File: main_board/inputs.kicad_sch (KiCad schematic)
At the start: 49 parts, among them J16 3.5mm Jack, J17 3.5mm Jack, U10 TLV2172IDR, U11 MCP3021, U12 TLV2172IDR, U13 MCP3021, U19 TLV2172IDR

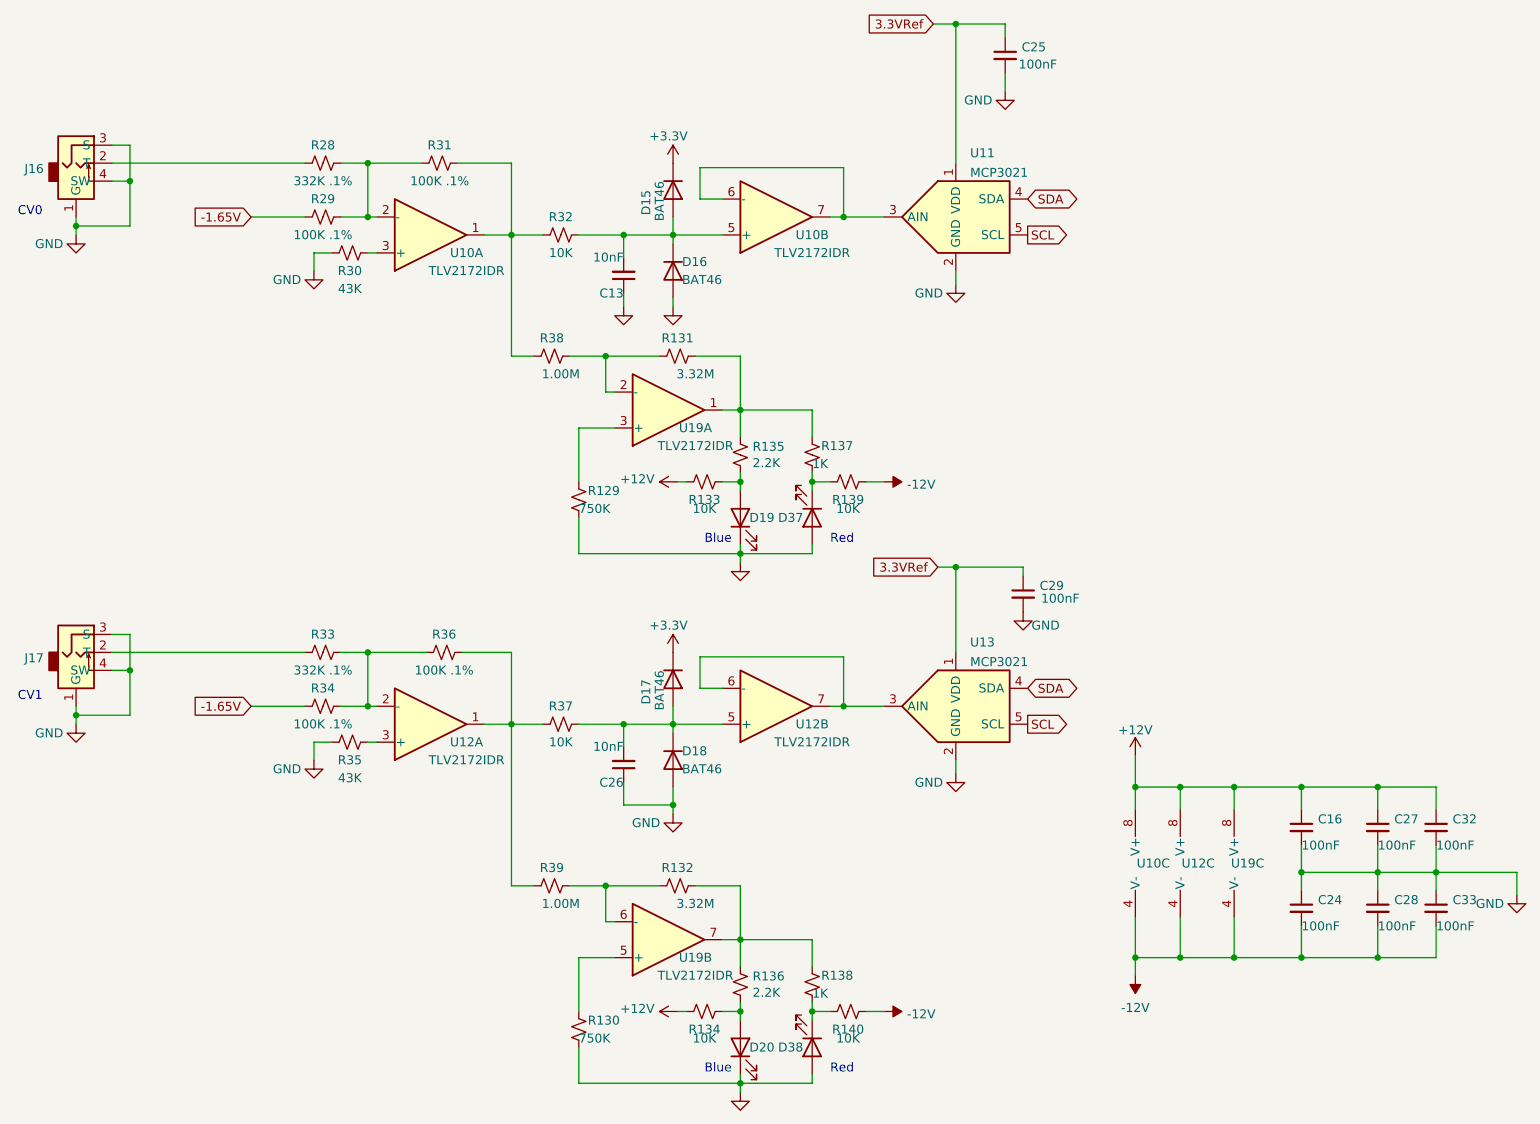
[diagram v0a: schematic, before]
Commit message: Version 0.03
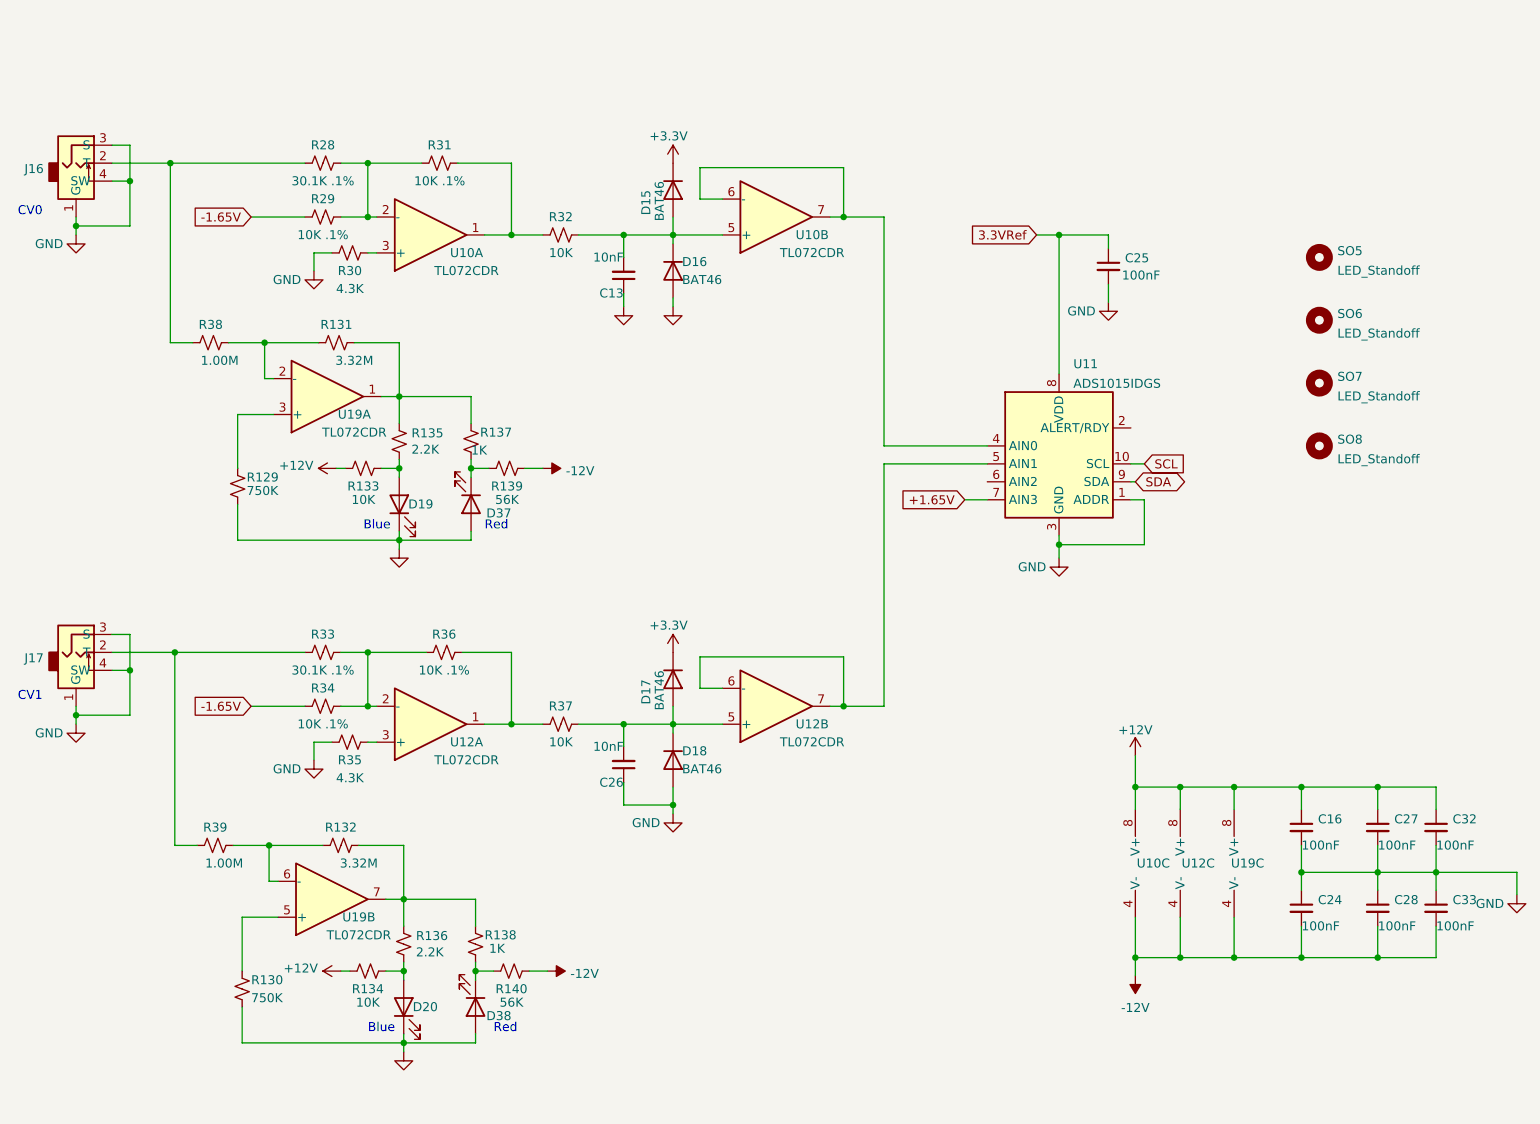
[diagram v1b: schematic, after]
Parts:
- removed C29: 100nF, Capacitor_SMD:C_0805_2012Metric_Pad1.18x1.45mm_HandSolder, symbol Device:C_Small
- removed U11, U13: MCP3021, Package_TO_SOT_SMD:TSOT-23-5_HandSoldering, symbol greenface:MCP3021
- added SO5, SO6, SO7, SO8: LED_Standoff, symbol greenface:LED_Standoff
- added U11: ADS1015IDGS, Package_SO:TSSOP-10_3x3mm_P0.5mm, symbol Analog_ADC:ADS1015IDGS
- R139, R140: value 10K -> 56K;  LCSC Part # C138260 -> C137420; Digi-Key Part 13-RC0805JR-1010KLCT-ND -> 311-56KARCT-ND
- R28, R33: value 332K .1% -> 30.1K .1%;  LCSC Part # C228750 -> C374678
- R29, R31, R34, R36: value 100K .1% -> 10K .1%;  LCSC Part # C122537 -> C406725; Digi-Key Part YAG1759CT-ND -> (none)
- R30, R35: value 43K -> 4.3K;  LCSC Part # C137429 -> C229218
- U10, U12, U19: value TLV2172IDR -> TL072CDR;  LCSC Part # C129149 -> C67473
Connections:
- net 3.3VRef: now also U11.8 (VDD)
- net GND: now also U11.1 (ADDR), U11.3 (GND)
- net SCL: now also U11.10 (SCL)
- net SDA: now also U11.9 (SDA)
- net at U10.6 (-), U10.7: now also U11.4 (AIN0)
- net at R31.1, R32.2, U10.1: no longer R38.1
- net at R36.1, R37.2, U12.1: no longer R39.1
- net at J16.2 (T), R28.2: now also R38.1
- net at J17.2 (T), R33.2: now also R39.1
- net at U12.6 (-), U12.7: now also U11.5 (AIN1)
- new net +1.65V: U11.7 (AIN3)
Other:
- moved on the sheet: C25, D19, D20, D37, D38, R129, R130, R131, R132, R133, R134, R135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
